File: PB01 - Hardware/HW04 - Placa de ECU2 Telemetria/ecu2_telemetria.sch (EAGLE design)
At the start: 24 parts, among them IC1 LM358N, X1 DAC, X2 COMB 1, X3 COMB 2, X4 MODULE CAN, X5 22-23-2041, X7 FORÇA

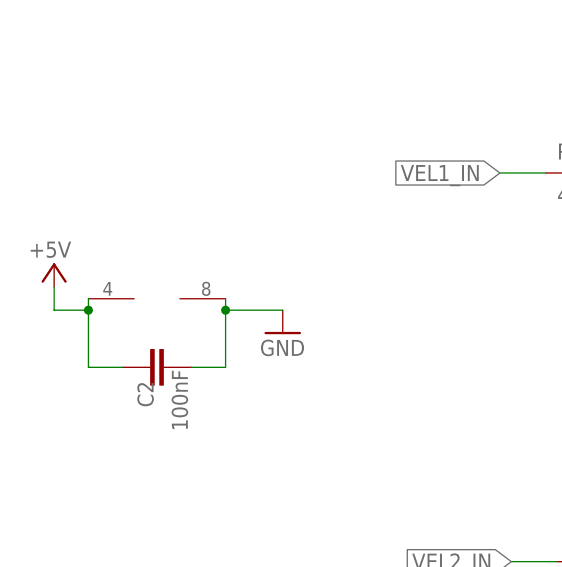
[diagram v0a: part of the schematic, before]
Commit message: Placa de AV 2.0
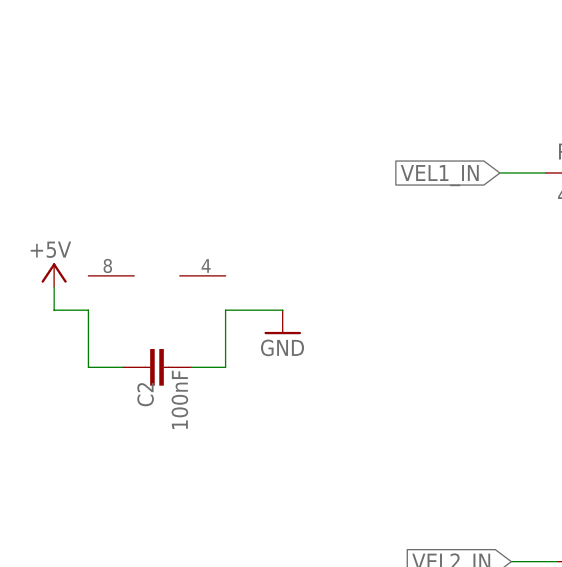
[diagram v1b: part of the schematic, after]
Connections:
- net +5V: no longer IC1P.V-
- net GND: no longer IC1P.V+
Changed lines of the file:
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@@
 <grid distance="0.05" unitdist="inch" unit="inch" style="lines" multiple="1" display="no" altdistance="0.01" altunitdist="inch" altunit="inch"/>
 <layers>
-<layer number="1" name="Top" color="4" fill="1" visible="yes" active="no"/>
-<layer number="2" name="Route2" color="1" fill="3" visible="yes" active="no"/>
-<layer number="3" name="Route3" color="4" fill="3" visible="yes" active="no"/>
-<layer number="4" name="Route4" color="1" fill="4" visible="yes" active="no"/>
-<layer number="5" name="Route5" color="4" fill="4" visible="yes" active="no"/>
-<layer number="6" name="Route6" color="1" fill="8" visible="yes" active="no"/>
-<layer number="7" name="Route7" color="4" fill="8" visible="yes" active="no"/>
-<layer number="8" name="Route8" color="1" fill="2" visible="yes" active="no"/>
-<layer number="9" name="Route9" color="4" fill="2" visible="yes" active="no"/>
-<layer number="10" name="Route10" color="1" fill="7" visible="yes" active="no"/>
-<layer number="11" name="Route11" color="4" fill="7" visible="yes" active="no"/>
-<layer number="12" name="Route12" color="1" fill="5" visible="yes" active="no"/>
-<layer number="13" name="Route13" color="4" fill="5" visible="yes" active="no"/>
-<layer number="14" name="Route14" color="1" fill="6" visible="yes" active="no"/>
-<layer number="15" name="Route15" color="4" fill="6" visible="yes" active="no"/>
-<layer number="16" name="Bottom" color="1" fill="1" visible="yes" active="no"/>
-<layer number="17" name="Pads" color="2" fill="1" visible="yes" active="no"/>
-<layer number="18" name="Vias" color="2" fill="1" visible="yes" active="no"/>
-<layer number="19" name="Unrouted" color="6" fill="1" visible="yes" active="no"/>
-<layer number="20" name="Dimension" color="24" fill="1" visible="yes" active="no"/>
-<layer number="21" name="tPlace" color="7" fill="1" visible="yes" active="no"/>
-<layer number="22" name="bPlace" color="7" fill="1" visible="yes" active="no"/>
-<layer number="23" name="tOrigins" color="15" fill="1" visible="yes" active="no"/>
-<layer number="24" name="bOrigins" color="15" fill="1" visible="yes" active="no"/>
-<layer number="25" name="tNames" color="7" fill="1" visible="yes" active="no"/>
-<layer number="26" name="bNames" color="7" fill="1" visible="yes" active="no"/>
-<layer number="27" name="tValues" color="7" fill="1" visible="yes" active="no"/>
-<layer number="28" name="bValues" color="7" fill="1" visible="yes" active="no"/>
+<layer number="1" name="Top" color="4" fill="1" visible="no" active="no"/>
+<layer number="2" name="Route2" color="1" fill="3" visible="no" active="no"/>
+<layer number="3" name="Route3" color="4" fill="3" visible="no" active="no"/>
+<layer number="4" name="Route4" color="1" fill="4" visible="no" active="no"/>
+<layer number="5" name="Route5" color="4" fill="4" visible="no" active="no"/>
+<layer number="6" name="Route6" color="1" fill="8" visible="no" active="no"/>
+<layer number="7" name="Route7" color="4" fill="8" visible="no" active="no"/>
+<layer number="8" name="Route8" color="1" fill="2" visible="no" active="no"/>
+<layer number="9" name="Route9" color="4" fill="2" visible="no" active="no"/>
+<layer number="10" name="Route10" color="1" fill="7" visible="no" active="no"/>
+<layer number="11" name="Route11" color="4" fill="7" visible="no" active="no"/>
+<layer number="12" name="Route12" color="1" fill="5" visible="no" active="no"/>
+<layer number="13" name="Route13" color="4" fill="5" visible="no" active="no"/>
+<layer number="14" name="Route14" color="1" fill="6" visible="no" active="no"/>
+<layer number="15" name="Route15" color="4" fill="6" visible="no" active="no"/>
+<layer number="16" name="Bottom" color="1" fill="1" visible="no" active="no"/>
+<layer number="17" name="Pads" color="2" fill="1" visible="no" active="no"/>
+<layer number="18" name="Vias" color="2" fill="1" visible="no" active="no"/>
+<layer number="19" name="Unrouted" color="6" fill="1" visible="no" active="no"/>
+<layer number="20" name="Dimension" color="24" fill="1" visible="no" active="no"/>
+<layer number="21" name="tPlace" color="7" fill="1" visible="no" active="no"/>
+<layer number="22" name="bPlace" color="7" fill="1" visible="no" active="no"/>
+<layer number="23" name="tOrigins" color="15" fill="1" visible="no" active="no"/>
+<layer number="24" name="bOrigins" color="15" fill="1" visible="no" active="no"/>
+<layer number="25" name="tNames" color="7" fill="1" visible="no" active="no"/>
+<layer number="26" name="bNames" color="7" fill="1" visible="no" active="no"/>
+<layer number="27" name="tValues" color="7" fill="1" visible="no" active="no"/>
+<layer number="28" name="bValues" color="7" fill="1" visible="no" active="no"/>
 <layer number="29" name="tStop" color="7" fill="3" visible="no" active="no"/>
 <layer number="30" name="bStop" color="7" fill="6" visible="no" active="no"/>
@@
 <layer number="35" name="tGlue" color="7" fill="4" visible="no" active="no"/>
 <layer number="36" name="bGlue" color="7" fill="5" visible="no" active="no"/>
-<layer number="37" name="tTest" color="7" fill="1" visible="yes" active="no"/>
-<layer number="38" name="bTest" color="7" fill="1" visible="yes" active="no"/>
+<layer number="37" name="tTest" color="7" fill="1" visible="no" active="no"/>
+<layer number="38" name="bTest" color="7" fill="1" visible="no" active="no"/>
 <layer number="39" name="tKeepout" color="4" fill="11" visible="no" active="no"/>
 <layer number="40" name="bKeepout" color="1" fill="11" visible="no" active="no"/>
@@
 <layer number="44" name="Drills" color="7" fill="1" visible="no" active="no"/>
 <layer number="45" name="Holes" color="7" fill="1" visible="no" active="no"/>
-<layer number="46" name="Milling" color="3" fill="1" visible="yes" active="no"/>
-<layer number="47" name="Measures" color="7" fill="1" visible="yes" active="no"/>
-<layer number="48" name="Document" color="7" fill="1" visible="yes" active="no"/>
-<layer number="49" name="Reference" color="7" fill="1" visible="yes" active="no"/>
-<layer number="50" name="dxf" color="7" fill="1" visible="yes" active="no"/>
-<layer number="51" name="tDocu" color="7" fill="1" visible="yes" active="no"/>
-<layer number="52" name="bDocu" color="7" fill="1" visible="yes" active="no"/>
-<layer number="53" name="tGND_GNDA" color="7" fill="9" visible="yes" active="no"/>
-<layer number="54" name="bGND_GNDA" color="1" fill="9" visible="yes" active="no"/>
-<layer number="56" name="wert" color="3" fill="1" visible="yes" active="no"/>
-<layer number="57" name="tCAD" color="7" fill="1" visible="yes" active="no"/>
-<layer number="59" name="tCarbon" color="7" fill="1" visible="yes" active="no"/>
-<layer number="60" name="bCarbon" color="7" fill="1" visible="yes" active="no"/>
+<layer number="46" name="Milling" color="3" fill="1" visible="no" active="no"/>
+<layer number="47" name="Measures" color="7" fill="1" visible="no" active="no"/>
+<layer number="48" name="Document" color="7" fill="1" visible="no" active="no"/>
+<layer number="49" name="Reference" color="7" fill="1" visible="no" active="no"/>
+<layer number="50" name="dxf" color="7" fill="1" visible="no" active="no"/>
+<layer number="51" name="tDocu" color="7" fill="1" visible="no" active="no"/>
+<layer number="52" name="bDocu" color="7" fill="1" visible="no" active="no"/>
+<layer number="53" name="tGND_GNDA" color="7" fill="9" visible="no" active="no"/>
+<layer number="54" name="bGND_GNDA" color="1" fill="9" visible="no" active="no"/>
+<layer number="56" name="wert" color="3" fill="1" visible="no" active="no"/>
+<layer number="57" name="tCAD" color="7" fill="1" visible="no" active="no"/>
+<layer number="59" name="tCarbon" color="7" fill="1" visible="no" active="no"/>
+<layer number="60" name="bCarbon" color="7" fill="1" visible="no" active="no"/>
 <layer number="88" name="SimResults" color="9" fill="1" visible="yes" active="yes"/>
 <layer number="89" name="SimProbes" color="9" fill="1" visible="yes" active="yes"/>
@@
 <instance part="IC1" gate="A" x="-95.25" y="83.82"/>
 <instance part="IC1" gate="B" x="-99.06" y="38.1"/>
-<instance part="IC1" gate="P" x="-173.99" y="69.85" rot="R270"/>
+<instance part="IC1" gate="P" x="-173.99" y="72.39" rot="R90"/>
 <instance part="SV8" gate="G$1" x="123.19" y="130.81" rot="R180"/>
 <instance part="P+8" gate="1" x="113.03" y="142.24" smashed="yes">
@@
 <wire x1="-166.37" y1="68.58" x2="-160.02" y2="68.58" width="0.1524" layer="91"/>
 <pinref part="C2" gate="G$1" pin="1"/>
-<pinref part="IC1" gate="P" pin="V+"/>
-<wire x1="-166.37" y1="69.85" x2="-166.37" y2="68.58" width="0.1524" layer="91"/>
-<junction x="-166.37" y="68.58"/>
 </segment>
 <segment>
@@
 <wire x1="-185.42" y1="68.58" x2="-185.42" y2="71.12" width="0.1524" layer="91"/>
 <pinref part="C2" gate="G$1" pin="2"/>
-<pinref part="IC1" gate="P" pin="V-"/>
-<wire x1="-181.61" y1="69.85" x2="-181.61" y2="68.58" width="0.1524" layer="91"/>
-<junction x="-181.61" y="68.58"/>
-</segment>
-<segment>
+</segment>
+<segment>
